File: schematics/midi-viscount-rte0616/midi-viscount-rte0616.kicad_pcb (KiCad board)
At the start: 2 copper layers, 17 parts, among them J1 Conn_02x07_Odd_Even, J10 Conn_01x01_Pin, J11 Conn_01x01_Pin, J12 Conn_01x01_Pin, J13 Conn_01x01_Pin, J2 Conn_01x01_Pin, J3 Conn_01x01_Pin, J4 Conn_01x01_Pin, J5 Conn_01x01_Pin, J6 Conn_01x01_Pin, J7 Conn_01x01_Pin, J8 Conn_01x01_Pin, J9 Conn_01x01_Pin, U1 ProMicro

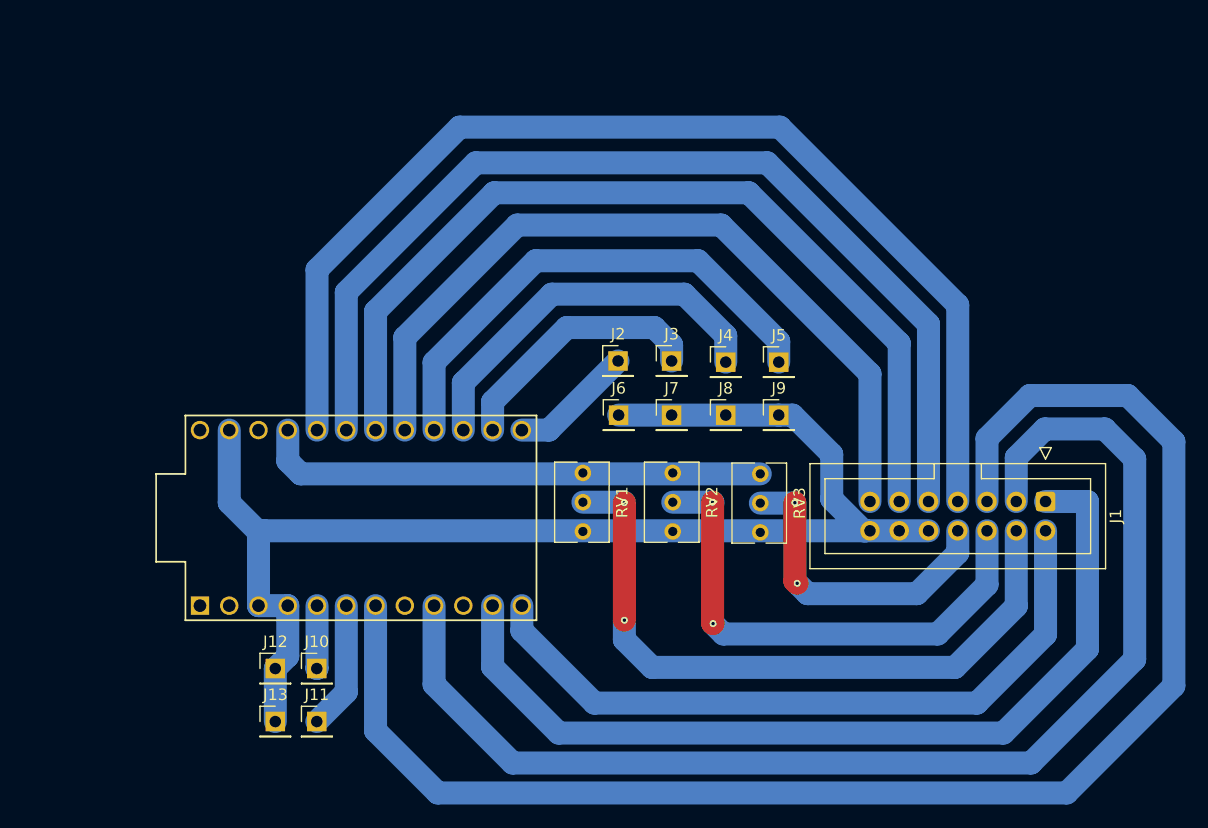
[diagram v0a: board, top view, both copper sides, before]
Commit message: Schematics rev1.1
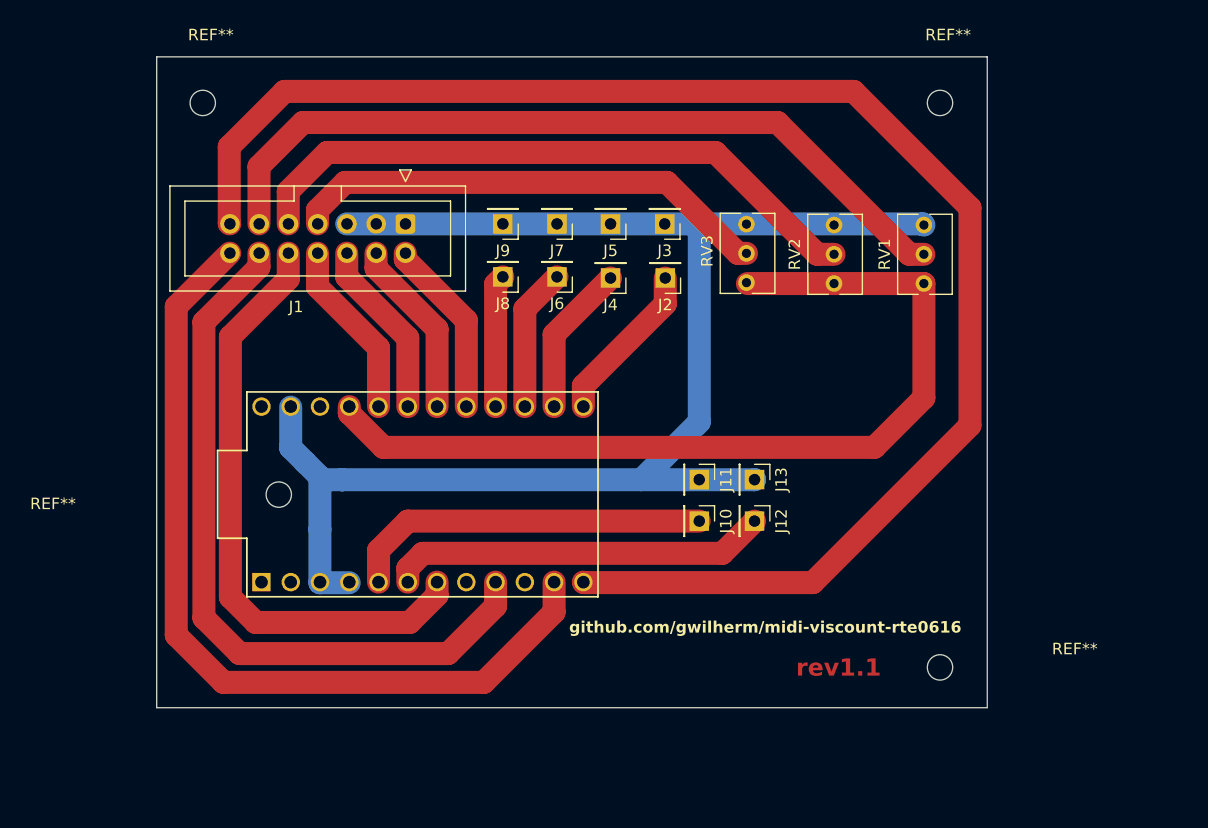
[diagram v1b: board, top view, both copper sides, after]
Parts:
- added REF**: MountingHole_2.2mm_M2_ISO7380, MountingHole:MountingHole_2.2mm_M2_ISO7380, F.Cu at (51.5, 62.7)
- added REF**: MountingHole_2.2mm_M2_ISO7380, MountingHole:MountingHole_2.2mm_M2_ISO7380, F.Cu at (108.9, 77.7)
- added REF**: MountingHole_2.2mm_M2_ISO7380, MountingHole:MountingHole_2.2mm_M2_ISO7380, F.Cu at (44.9, 28.7)
- added REF**: MountingHole_2.2mm_M2_ISO7380, MountingHole:MountingHole_2.2mm_M2_ISO7380, F.Cu at (108.9, 28.7)
- moved J1 60.6 mm to (62.5, 39.2)
- moved J13 46.6 mm to (92.8, 61.4), turned to -90 degrees
- moved J12 41.8 mm to (92.8, 65.0), turned to -90 degrees
- moved J11 40.3 mm to (88.0, 61.4), turned to -90 degrees
- moved RV1 39.8 mm to (107.5, 39.3), turned to 90 degrees
- moved J10 35.6 mm to (88.0, 65.0), turned to -90 degrees
- moved RV2 30.1 mm to (99.7, 39.3), turned to 90 degrees
- moved J9 29.1 mm to (71.0, 39.2), turned to 180 degrees
- moved RV3 26.8 mm to (92.1, 39.2), turned to 90 degrees
- moved J8 25.1 mm to (71.0, 43.8), turned to 180 degrees
- moved J7 22.1 mm to (75.7, 39.2), turned to 180 degrees
- moved J5 17.4 mm to (80.3, 39.2), turned to 180 degrees
- moved J3 17.1 mm to (85.0, 39.2), turned to 180 degrees
- moved J6 16.4 mm to (75.7, 43.8), turned to 180 degrees
- moved J4 8.94 mm to (80.3, 43.9), turned to 180 degrees
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- renumbered J12 to J11, J11 to J12, J6 to J3, J3 to J4, J7 to J5, J4 to J6, J8 to J7, J5 to J8
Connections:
- J1 pad 1: Net-(J1-Pin_1) -> Vseg4
- J1 pad 10: Vseg4 -> Net-(J1-Pin_10)
- J1 pad 11: Net-(J1-Pin_11) -> Vseg1
- J1 pad 12: Vseg4 -> Net-(J1-Pin_12)
- J1 pad 14: Vseg4 -> Net-(J1-Pin_14)
- J1 pad 3: Net-(J1-Pin_3) -> Vseg4
- J1 pad 4: Vseg1 -> Net-(J1-Pin_4)
- J1 pad 5: Net-(J1-Pin_5) -> Vseg4
- J1 pad 6: Vseg2 -> Net-(J1-Pin_6)
- J1 pad 7: Net-(J1-Pin_7) -> VSeg3
- J1 pad 8: VSeg3 -> Net-(J1-Pin_8)
- J1 pad 9: Net-(J1-Pin_9) -> Vseg2
- U1 pad 11: Net-(J1-Pin_1) -> Net-(J1-Pin_14)
- U1 pad 12: Net-(J1-Pin_2) -> Net-(J1-Pin_13)
- U1 pad 17: Net-(J1-Pin_13) -> Net-(J1-Pin_2)
- U1 pad 18: Net-(J1-Pin_11) -> Net-(J1-Pin_4)
- U1 pad 19: Net-(J1-Pin_9) -> Net-(J1-Pin_6)
- U1 pad 20: Net-(J1-Pin_7) -> Net-(J1-Pin_8)
- U1 pad 7: Net-(J1-Pin_5) -> Net-(J1-Pin_10)
- U1 pad 9: Net-(J1-Pin_3) -> Net-(J1-Pin_12)
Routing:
- net Net-(J1-Pin_5): track 132.3 -> 0.00 mm
- net Net-(J1-Pin_3): track 107.8 -> 0.00 mm
- net Net-(J1-Pin_7): track 98.1 -> 0.00 mm
- net Net-(J1-Pin_9): track 88.4 -> 0.00 mm
- net Net-(J1-Pin_11): track 79.2 -> 0.00 mm
- net Net-(J1-Pin_1): track 78.8 -> 0.00 mm
- net Net-(J1-Pin_14): track 0.00 -> 74.7 mm
- net Net-(J1-Pin_13): track 68.9 -> 135.3 mm
- net Net-(J1-Pin_12): track 0.00 -> 64.0 mm
- net Net-(J1-Pin_10): track 0.00 -> 52.9 mm
- net Net-(J1-Pin_2): track 61.7 -> 15.5 mm
- net Net-(U1-VCC): track 44.2 -> 78.7 mm
- net Net-(J8-Pin_1): track 44.2 -> 11.5 mm
- net Net-(J10-Pin_1): track 5.47 -> 31.7 mm
- net Net-(J12-Pin_1): track 11.1 -> 33.0 mm
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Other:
- board outline added: 72.1 x 56.5 mm
- board text added: "github.com/gwilherm/midi-viscount-rte0616"
- board text added: "rev1.1"
